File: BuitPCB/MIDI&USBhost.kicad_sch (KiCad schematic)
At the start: 10 parts, among them J1 MIDI IN, J2 MIDI OUT, J3 USB HOST, U2 6N138

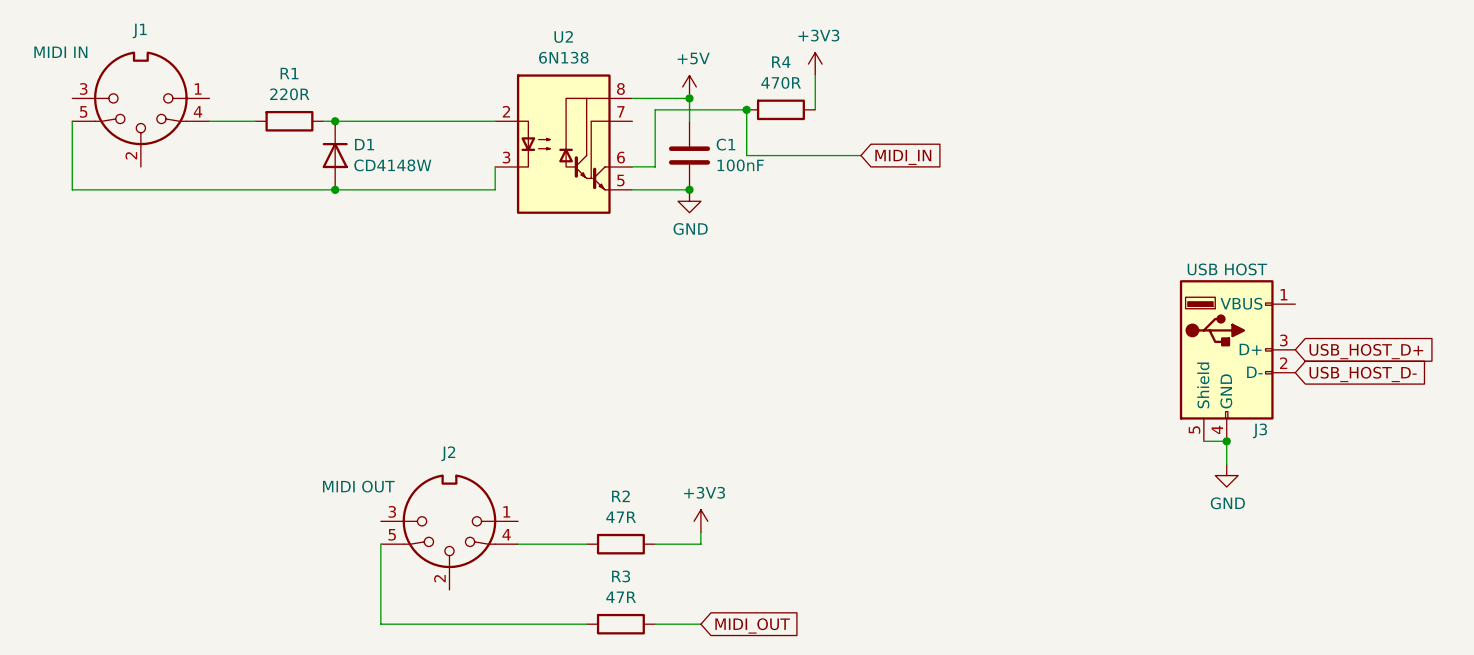
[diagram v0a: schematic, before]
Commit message: Updated almost to final 0.1 version
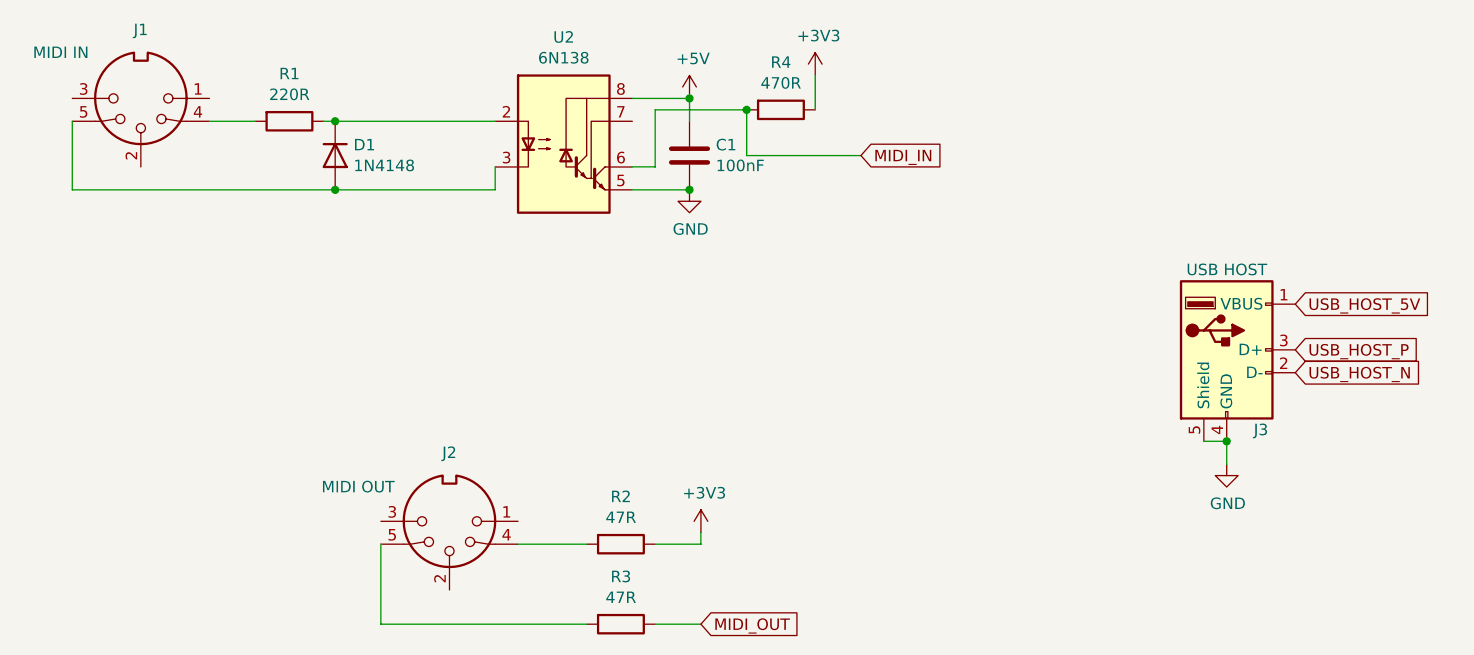
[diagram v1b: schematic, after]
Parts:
- D1: value CD4148W -> 1N4148
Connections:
- net USB_HOST_5V: now reaches J3.1 (VBUS)
- net USB_HOST_D+ renamed USB_HOST_P
- net USB_HOST_D- renamed USB_HOST_N
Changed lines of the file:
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@@
     )
   )
-  (global_label "USB_HOST_D+" (shape input) (at 236.22 91.44 0) (fields_autoplaced)
+  (global_label "USB_HOST_5V" (shape input) (at 236.22 86.36 0) (fields_autoplaced)
+    (effects (font (size 1.27 1.27)) (justify left))
+    (property "Intersheet References" "${INTERSHEET_REFS}" (id 0) (at 302.26 200.66 0)
+      (effects (font (size 1.27 1.27)) hide)
+    )
+  )
+  (global_label "MIDI_IN" (shape input) (at 187.96 69.85 0) (fields_autoplaced)
     (effects (font (size 1.27 1.27)) (justify left))
     (property "Intersheet References" "${INTERSHEET_REFS}" (id 0) (at 0 0 0)
@@
     )
   )
-  (global_label "MIDI_IN" (shape input) (at 187.96 69.85 0) (fields_autoplaced)
-    (effects (font (size 1.27 1.27)) (justify left))
-    (property "Intersheet References" "${INTERSHEET_REFS}" (id 0) (at 0 0 0)
-      (effects (font (size 1.27 1.27)) hide)
-    )
-  )
-  (global_label "USB_HOST_D-" (shape input) (at 236.22 93.98 0) (fields_autoplaced)
-    (effects (font (size 1.27 1.27)) (justify left))
-    (property "Intersheet References" "${INTERSHEET_REFS}" (id 0) (at 0 0 0)
-      (effects (font (size 1.27 1.27)) hide)
+  (global_label "USB_HOST_N" (shape input) (at 236.22 93.98 0) (fields_autoplaced)
+    (effects (font (size 1.27 1.27)) (justify left))
+    (property "Intersheet References" "${INTERSHEET_REFS}" (id 0) (at 250.458 94.0594 0)
+      (effects (font (size 1.27 1.27)) (justify left) hide)
+    )
+  )
+  (global_label "USB_HOST_P" (shape input) (at 236.22 91.44 0) (fields_autoplaced)
+    (effects (font (size 1.27 1.27)) (justify left))
+    (property "Intersheet References" "${INTERSHEET_REFS}" (id 0) (at 250.3975 91.5194 0)
+      (effects (font (size 1.27 1.27)) (justify left) hide)
     )
   )
@@
       (effects (font (size 1.27 1.27)) (justify left))
     )
-    (property "Value" "CD4148W" (id 1) (at 131.572 70.993 90)
+    (property "Value" "1N4148" (id 1) (at 131.572 70.993 90)
       (effects (font (size 1.27 1.27)) (justify left))
     )
@@
     (pin "1")
   )
-  (symbol (lib_id "Connector:USB_A") (at 228.6 91.44 0)
+  (symbol (lib_id "Connector:USB_A") (at 228.6 91.44 0) (unit 1)
     (in_bom yes) (on_board yes)
     (property "Reference" "J3" (id 0) (at 232.41 100.33 0))
@@
     (pin "5")
   )
-  (symbol (lib_id "power:GND") (at 228.6 104.14 0)
+  (symbol (lib_id "power:GND") (at 228.6 104.14 0) (unit 1)
     (in_bom yes) (on_board yes)
     (property "Reference" "#PWR05" (id 0) (at 228.6 110.49 0)
